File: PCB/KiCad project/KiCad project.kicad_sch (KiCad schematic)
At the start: 7 parts, among them SW1 SW_Push, SW2 SW_Push, SW3 SW_Push, SW4 SW_Push, U1 XIAO-RP2040-DIP

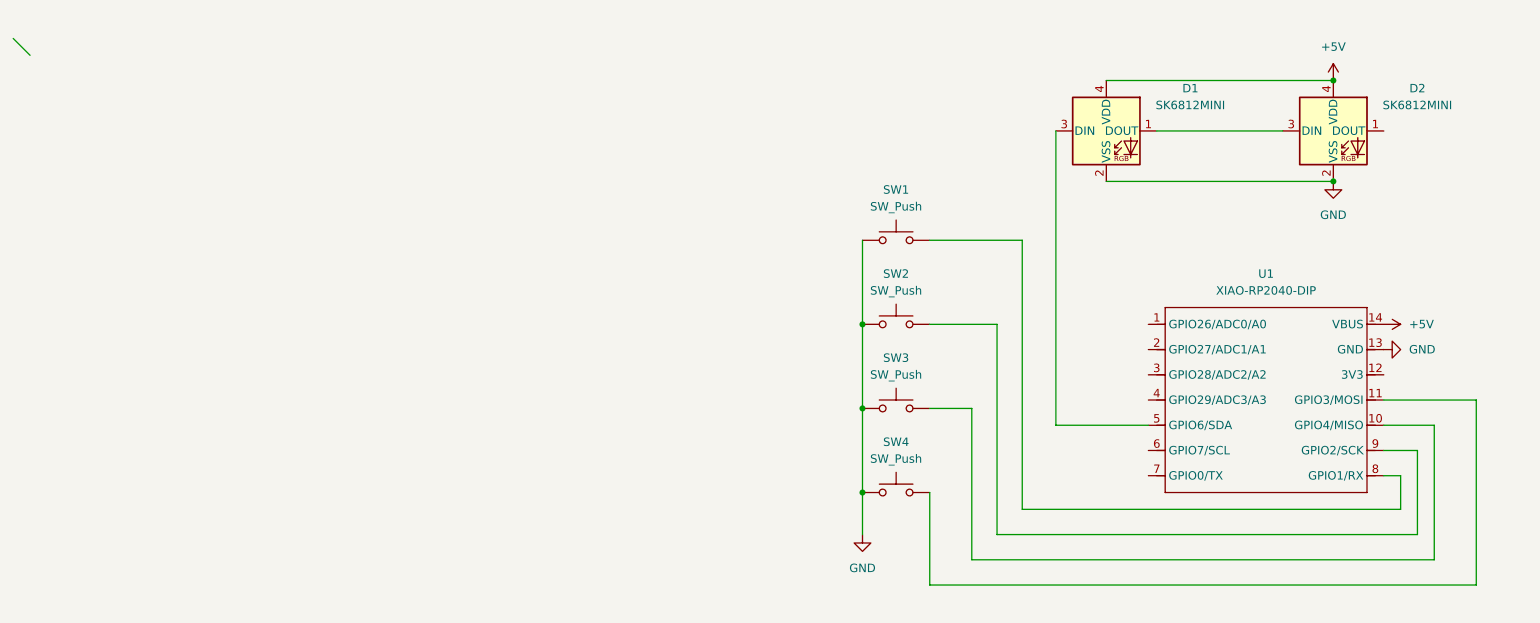
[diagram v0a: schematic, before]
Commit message: Add files via upload
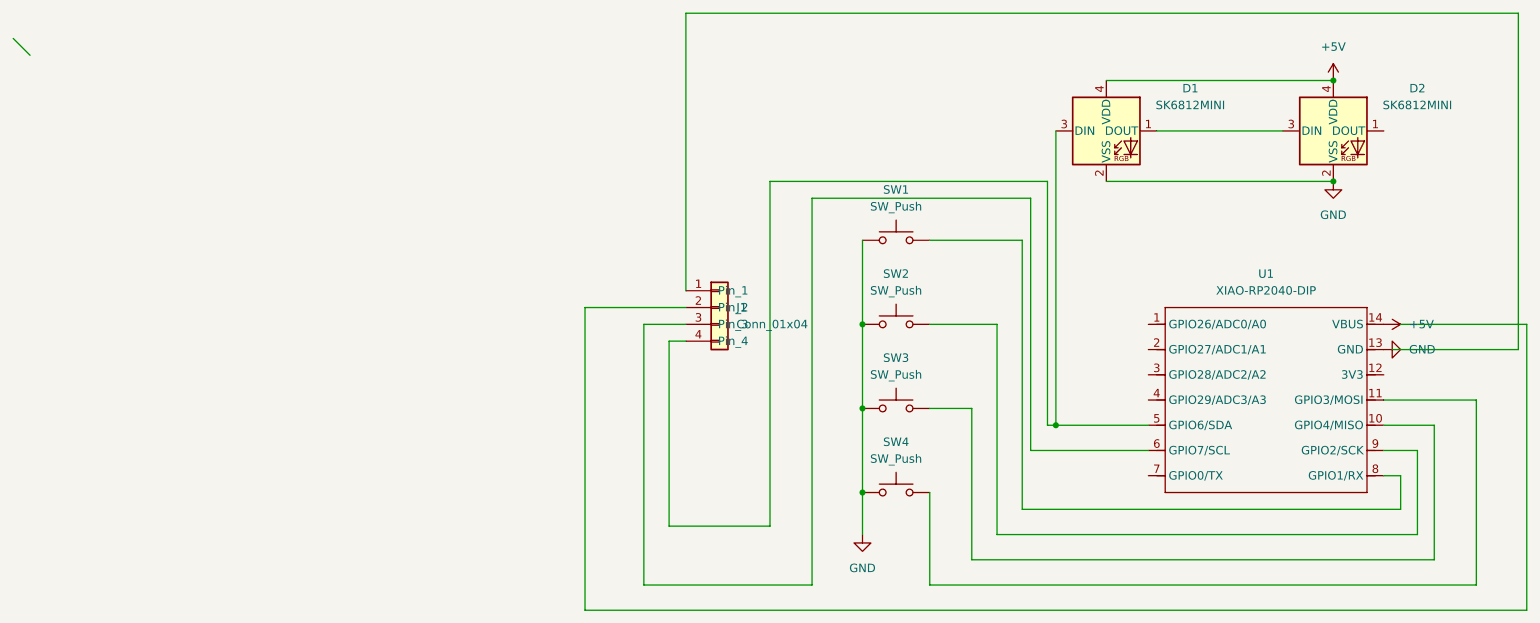
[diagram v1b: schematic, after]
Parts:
- added J1: Conn_01x04, Connector_PinHeader_2.54mm:PinHeader_1x04_P2.54mm_Vertical, symbol Connector_Generic:Conn_01x04
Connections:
- net at D1.3 (DIN), U1.5 (GPIO6/SDA): now also J1.4 (Pin_4)
- net at U1.6 (GPIO7/SCL): now also J1.3 (Pin_3)
